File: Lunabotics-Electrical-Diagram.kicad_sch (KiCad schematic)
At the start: 3 parts, among them J1 PDB_Mains, J2 PDB_CAN, J3 Talon

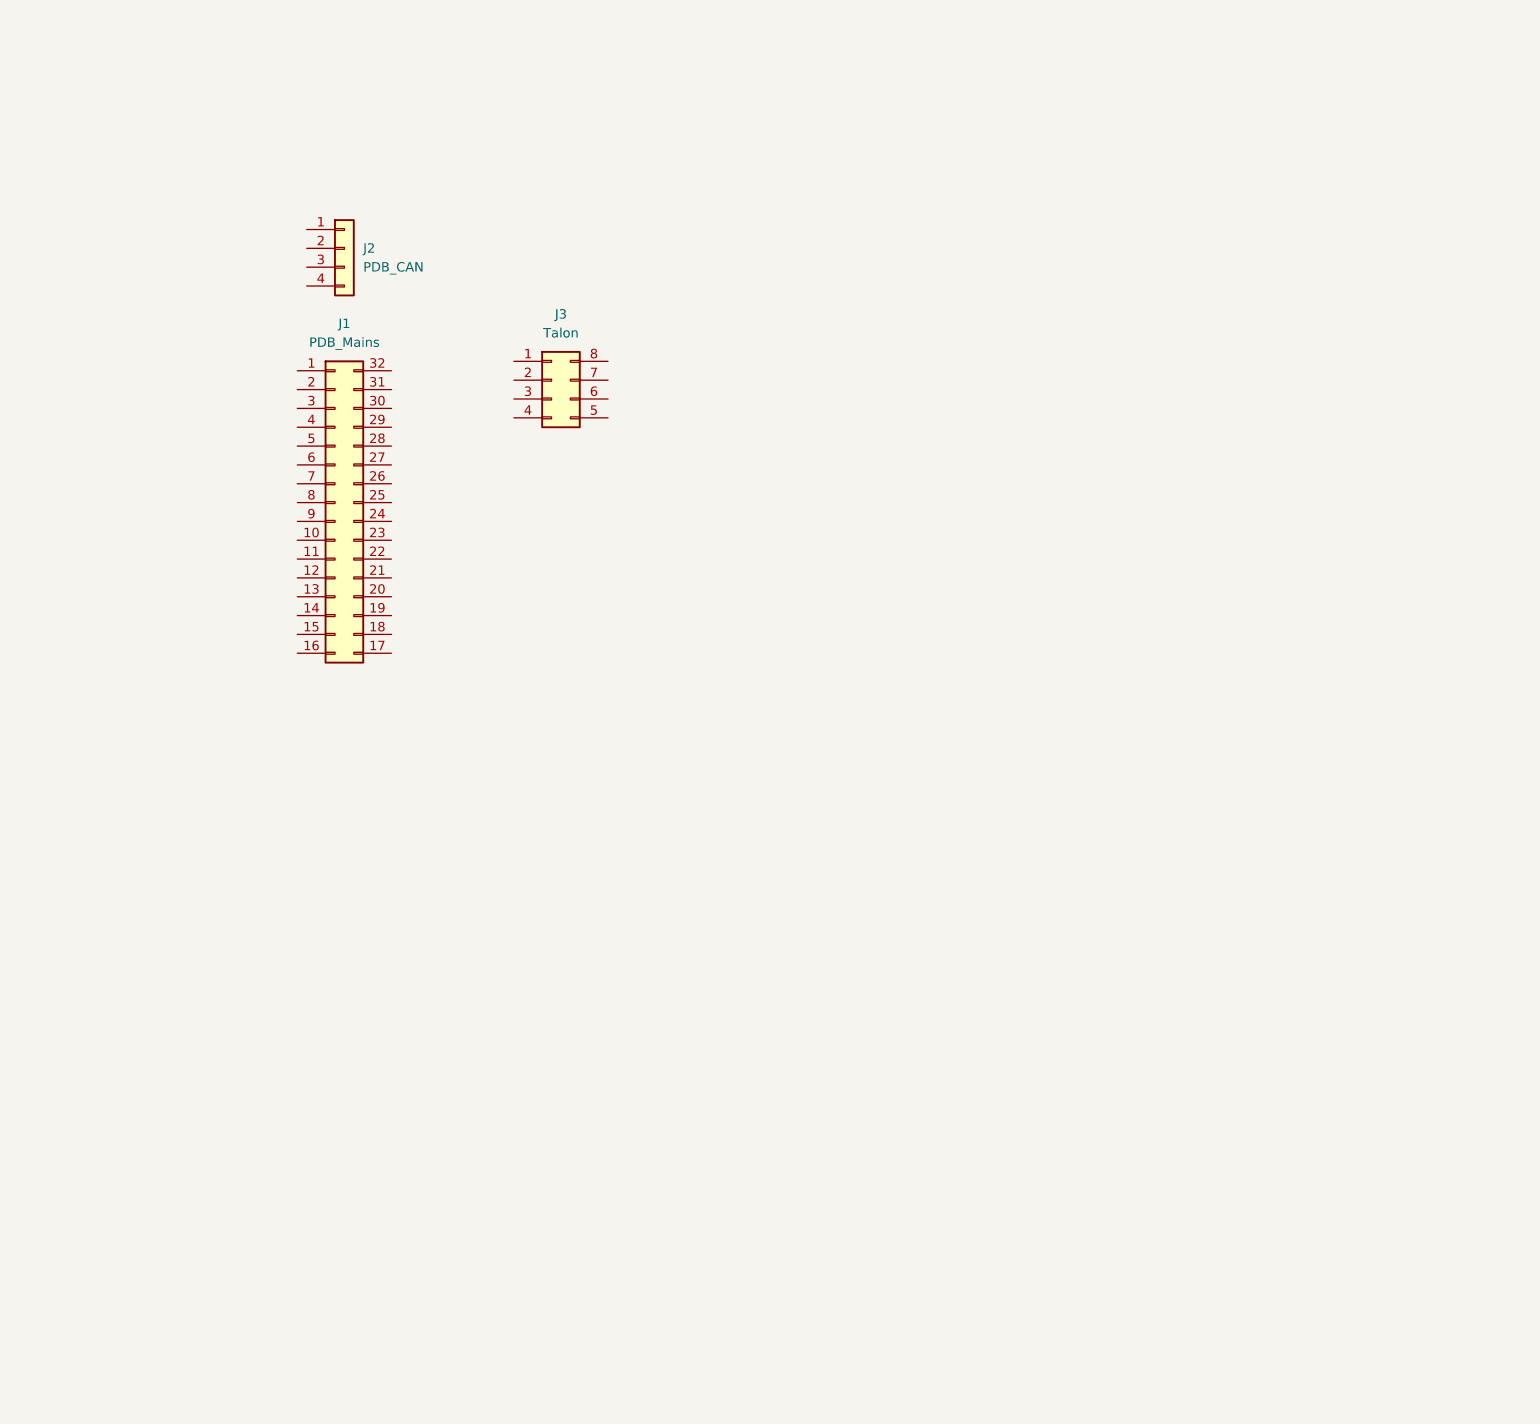
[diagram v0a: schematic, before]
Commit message: Finsihed V1
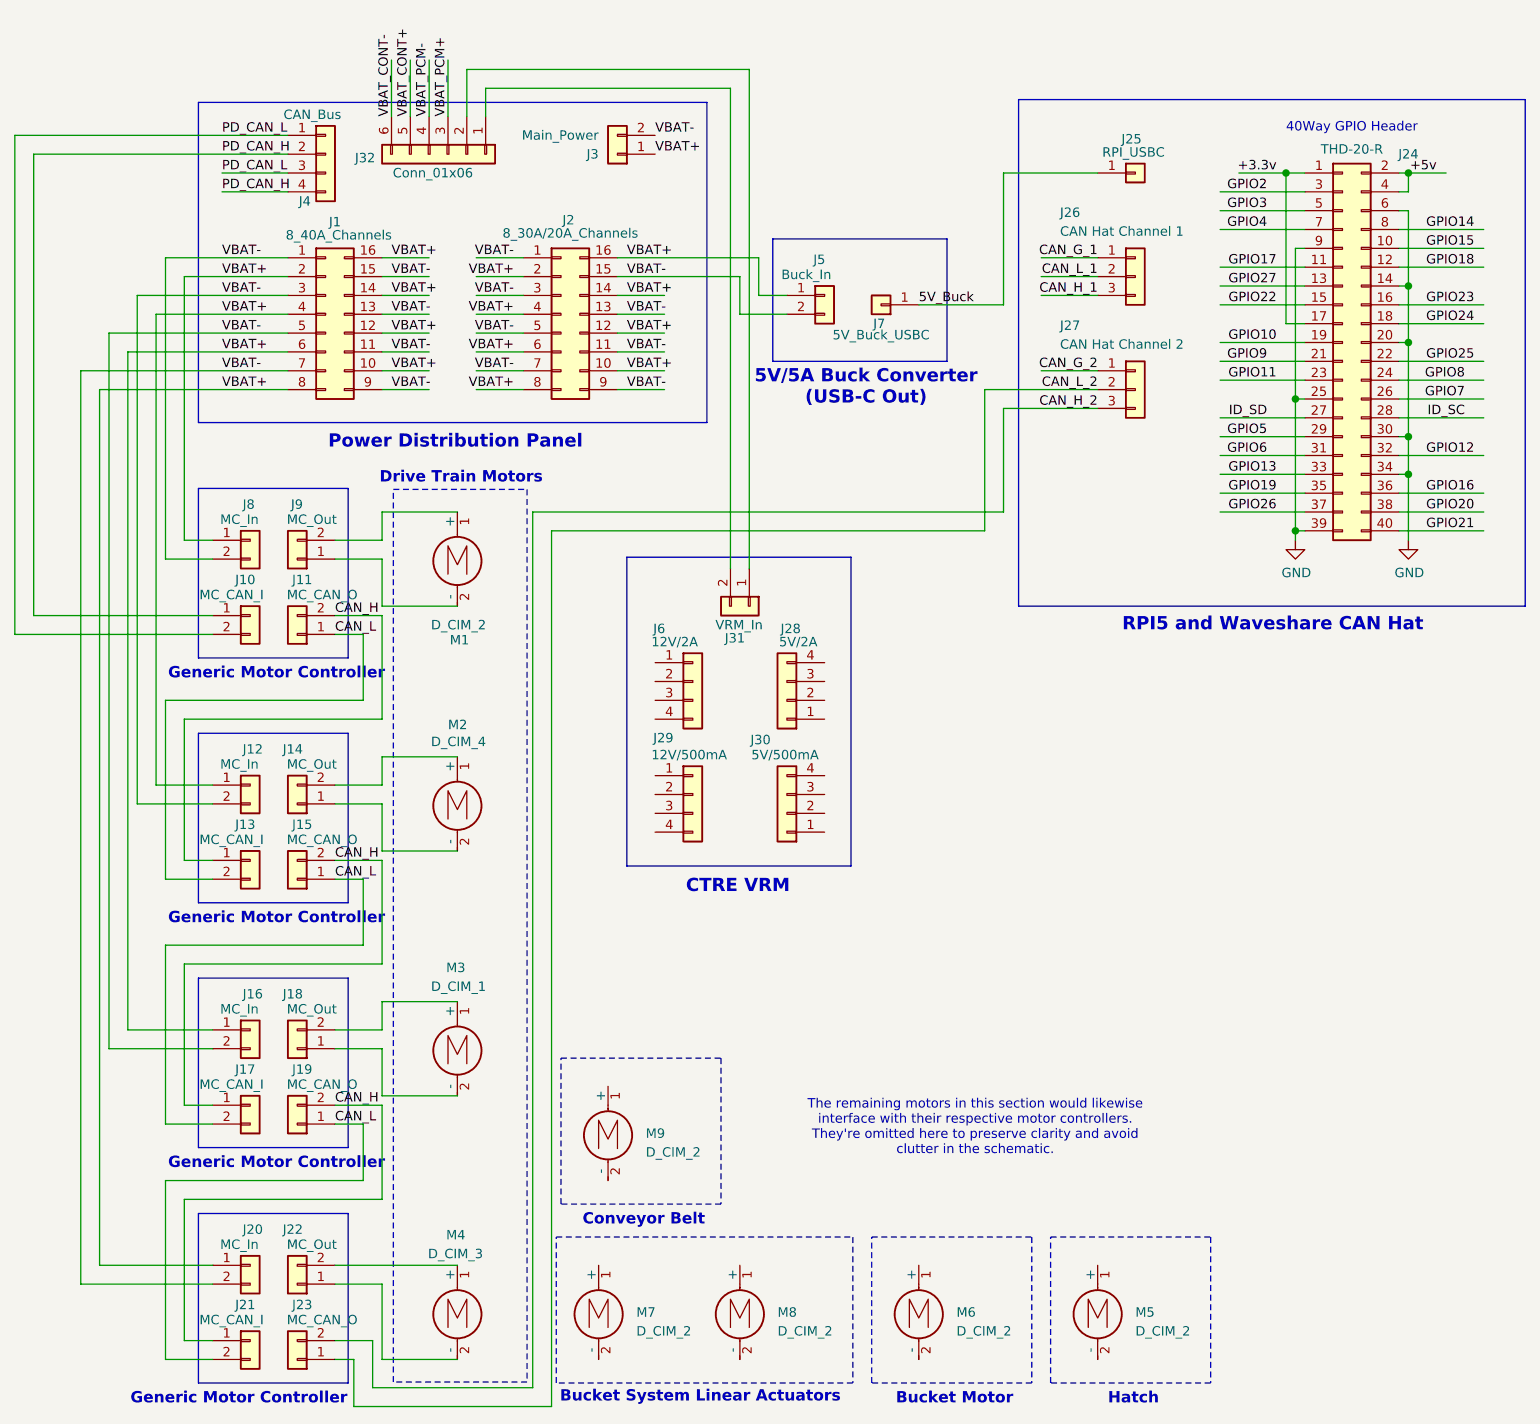
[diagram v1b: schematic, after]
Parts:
- removed J1: PDB_Mains, symbol Connector_Generic:Conn_02x16_Counter_Clockwise
- removed J2: PDB_CAN, symbol Connector_Generic:Conn_01x04
- removed J3: Talon, symbol Connector_Generic:Conn_02x04_Counter_Clockwise
- added J1: 8_40A_Channels, symbol Connector_Generic:Conn_02x08_Counter_Clockwise
- added J10, J13, J17, J21: MC_CAN_I, symbol Connector_Generic:Conn_01x02
- added J11, J15, J19, J23: MC_CAN_O, symbol Connector_Generic:Conn_01x02
- added J12, J16, J20, J8: MC_In, symbol Connector_Generic:Conn_01x02
- added J14, J18, J22, J9: MC_Out, symbol Connector_Generic:Conn_01x02
- added J2: 8_30A/20A_Channels, symbol Connector_Generic:Conn_02x08_Counter_Clockwise
- added J24: THD-20-R, Connector_PinHeader_2.54mm:PinHeader_2x20_P2.54mm_Vertical, symbol Connector_Generic:Conn_02x20_Odd_Even
- added J25: RPI_USBC, symbol Connector_Generic:Conn_01x01
- added J26: CAN Hat Channel 1, symbol Connector_Generic:Conn_01x03
- added J27: CAN Hat Channel 2, symbol Connector_Generic:Conn_01x03
- added J28: 5V/2A, symbol Connector_Generic:Conn_01x04
- added J29: 12V/500mA, symbol Connector_Generic:Conn_01x04
- added J3: Main_Power, symbol Connector_Generic:Conn_01x02
- added J30: 5V/500mA, symbol Connector_Generic:Conn_01x04
- added J31: VRM_In, symbol Connector_Generic:Conn_01x02
- added J32: Conn_01x06, symbol Connector_Generic:Conn_01x06
- added J4: CAN_Bus, symbol Connector_Generic:Conn_01x04
- added J5: Buck_In, symbol Connector_Generic:Conn_01x02
- added J6: 12V/2A, symbol Connector_Generic:Conn_01x04
- added J7: 5V_Buck_USBC, symbol Connector_Generic:Conn_01x01
- added M1, M5, M6, M7, M8, M9: D_CIM_2, symbol Motor:Motor_DC
- added M2: D_CIM_4, symbol Motor:Motor_DC
- added M3: D_CIM_1, symbol Motor:Motor_DC
- added M4: D_CIM_3, symbol Motor:Motor_DC
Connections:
- new net: J22.2 (Pin_2), M4.1 (+)
- new net: J22.1 (Pin_1), M4.2 (-)
- new net: J9.2 (Pin_2), M1.1 (+)
- new net: J9.1 (Pin_1), M1.2 (-)
- new net: J31.2 (Pin_2), J32.1 (Pin_1)
- new net: J31.1 (Pin_1), J32.2 (Pin_2)
- new net: J14.1 (Pin_1), M2.2 (-)
- new net: J14.2 (Pin_2), M2.1 (+)
- new net: J18.1 (Pin_1), M3.2 (-)
- new net: J18.2 (Pin_2), M3.1 (+)
- new net +3.3v: J24.1 (Pin_1), J24.17 (Pin_17)
- new net +5v: J24.2 (Pin_2), J24.4 (Pin_4)
- new net 5V_Buck: J25.1 (Pin_1), J7.1 (Pin_1)
- new net CAN_G_1: J26.1 (Pin_1)
- new net CAN_G_2: J27.1 (Pin_1)
- new net CAN_H: J11.2 (Pin_2), J13.1 (Pin_1), J15.2 (Pin_2), J17.1 (Pin_1), J19.2 (Pin_2), J21.1 (Pin_1)
- new net CAN_H_1: J26.3 (Pin_3)
- new net CAN_H_2: J23.2 (Pin_2), J27.3 (Pin_3)
- new net CAN_L: J11.1 (Pin_1), J13.2 (Pin_2), J15.1 (Pin_1), J17.2 (Pin_2), J19.1 (Pin_1), J21.2 (Pin_2)
- new net CAN_L_1: J26.2 (Pin_2)
- new net CAN_L_2: J23.1 (Pin_1), J27.2 (Pin_2)
- new net GND: J24.14 (Pin_14), J24.20 (Pin_20), J24.25 (Pin_25), J24.30 (Pin_30), J24.34 (Pin_34), J24.39 (Pin_39), J24.6 (Pin_6), J24.9 (Pin_9)
- new net GPIO10: J24.19 (Pin_19)
- new net GPIO11: J24.23 (Pin_23)
- new net GPIO12: J24.32 (Pin_32)
- new net GPIO13: J24.33 (Pin_33)
- new net GPIO14: J24.8 (Pin_8)
- new net GPIO15: J24.10 (Pin_10)
- new net GPIO16: J24.36 (Pin_36)
- new net GPIO17: J24.11 (Pin_11)
- new net GPIO18: J24.12 (Pin_12)
- new net GPIO19: J24.35 (Pin_35)
- new net GPIO2: J24.3 (Pin_3)
- new net GPIO20: J24.38 (Pin_38)
- new net GPIO21: J24.40 (Pin_40)
- new net GPIO22: J24.15 (Pin_15)
- new net GPIO23: J24.16 (Pin_16)
- new net GPIO24: J24.18 (Pin_18)
- new net GPIO25: J24.22 (Pin_22)
- new net GPIO26: J24.37 (Pin_37)
- new net GPIO27: J24.13 (Pin_13)
- new net GPIO3: J24.5 (Pin_5)
- new net GPIO4: J24.7 (Pin_7)
- new net GPIO5: J24.29 (Pin_29)
- new net GPIO6: J24.31 (Pin_31)
- new net GPIO7: J24.26 (Pin_26)
- new net GPIO8: J24.24 (Pin_24)
- new net GPIO9: J24.21 (Pin_21)
- new net ID_SC: J24.28 (Pin_28)
- new net ID_SD: J24.27 (Pin_27)
- new net PD_CAN_H: J10.1 (Pin_1), J4.2 (Pin_2), J4.4 (Pin_4)
- new net PD_CAN_L: J10.2 (Pin_2), J4.1 (Pin_1), J4.3 (Pin_3)
- new net VBAT+: J1.10 (Pin_10), J1.12 (Pin_12), J1.14 (Pin_14), J1.16 (Pin_16), J1.2 (Pin_2), J1.4 (Pin_4), J1.6 (Pin_6), J1.8 (Pin_8), J12.1 (Pin_1), J16.1 (Pin_1), J2.10 (Pin_10), J2.12 (Pin_12), J2.14 (Pin_14), J2.16 (Pin_16), J2.2 (Pin_2), J2.4 (Pin_4), J2.6 (Pin_6), J2.8 (Pin_8), J20.1 (Pin_1), J3.1 (Pin_1), J5.1 (Pin_1), J8.1 (Pin_1)
- new net VBAT-: J1.1 (Pin_1), J1.11 (Pin_11), J1.13 (Pin_13), J1.15 (Pin_15), J1.3 (Pin_3), J1.5 (Pin_5), J1.7 (Pin_7), J1.9 (Pin_9), J12.2 (Pin_2), J16.2 (Pin_2), J2.1 (Pin_1), J2.11 (Pin_11), J2.13 (Pin_13), J2.15 (Pin_15), J2.3 (Pin_3), J2.5 (Pin_5), J2.7 (Pin_7), J2.9 (Pin_9), J20.2 (Pin_2), J3.2 (Pin_2), J5.2 (Pin_2), J8.2 (Pin_2)
- new net VBAT_CONT+: J32.5 (Pin_5)
- new net VBAT_CONT-: J32.6 (Pin_6)
- new net VBAT_PCM+: J32.3 (Pin_3)
- new net VBAT_PCM-: J32.4 (Pin_4)
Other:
- note added: "40Way GPIO Header"
- note added: "5V/5A Buck Converter (USB-C Out)"
- note added: "Bucket Motor"
- note added: "Bucket System Linear Actuators"
- note added: "CTRE VRM"
- note added: "Conveyor Belt"
- note added: "Drive Train Motors"
- note added: "Generic Motor Controller"
- note added: "Hatch"
- note added: "Power Distribution Panel"
- note added: "RPI5 and Waveshare CAN Hat"
- note added: "The remaining motors in this section would likewise interface with their respective motor controllers. They're omitted here to preserve clarity and avoid clutter in the schematic."
